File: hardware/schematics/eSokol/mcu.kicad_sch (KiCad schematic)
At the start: 12 parts, among them J1 DB25, J2 to HC-05, SW1 SW_LITTLE, U2 YAAJ_BluePill_SWD_Breakout, U3 TP4056, U9 TCRT5000

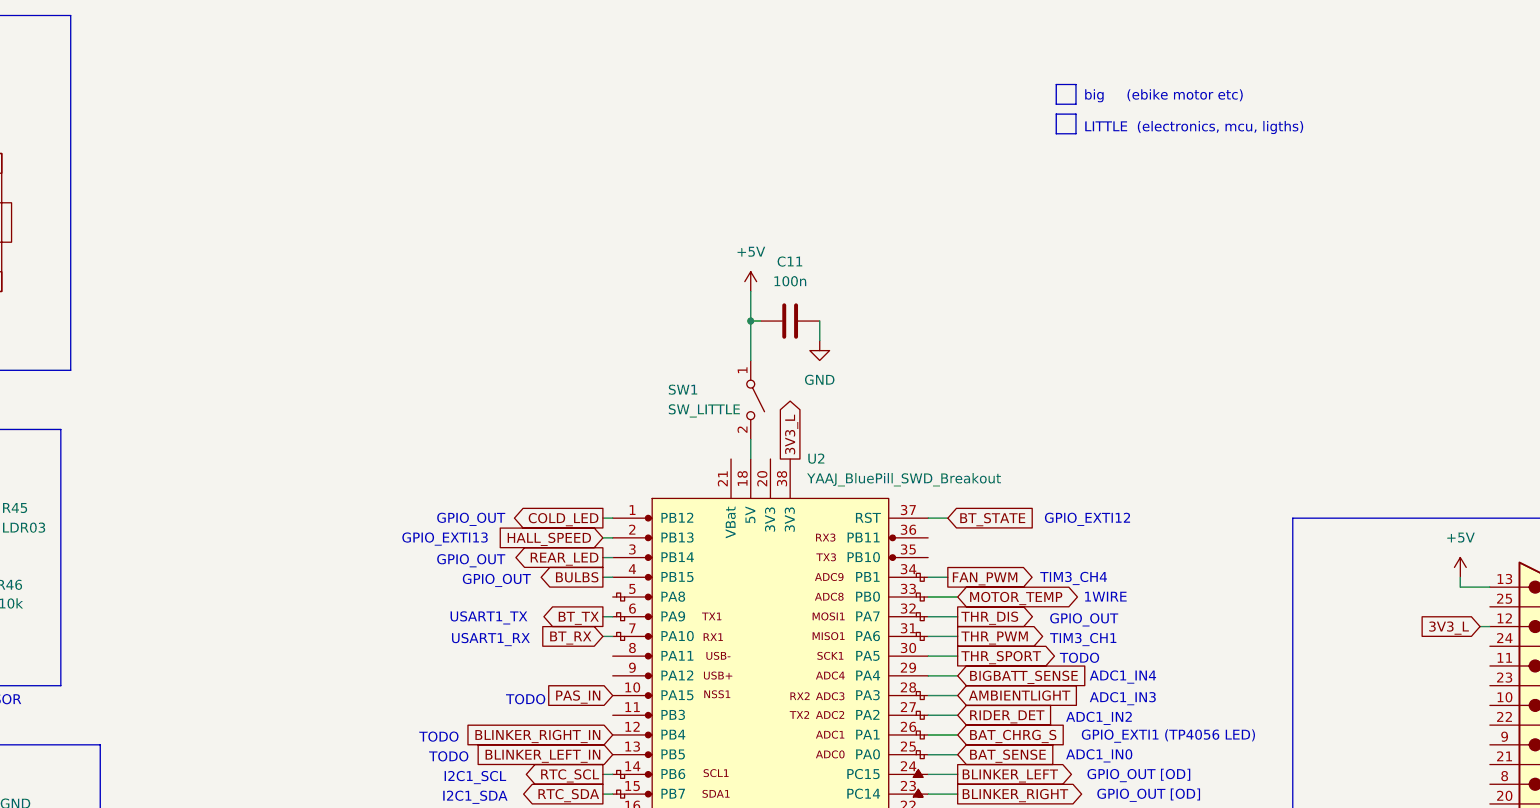
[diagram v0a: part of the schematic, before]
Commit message: WIP: update some schematics to reflect the newest design changes
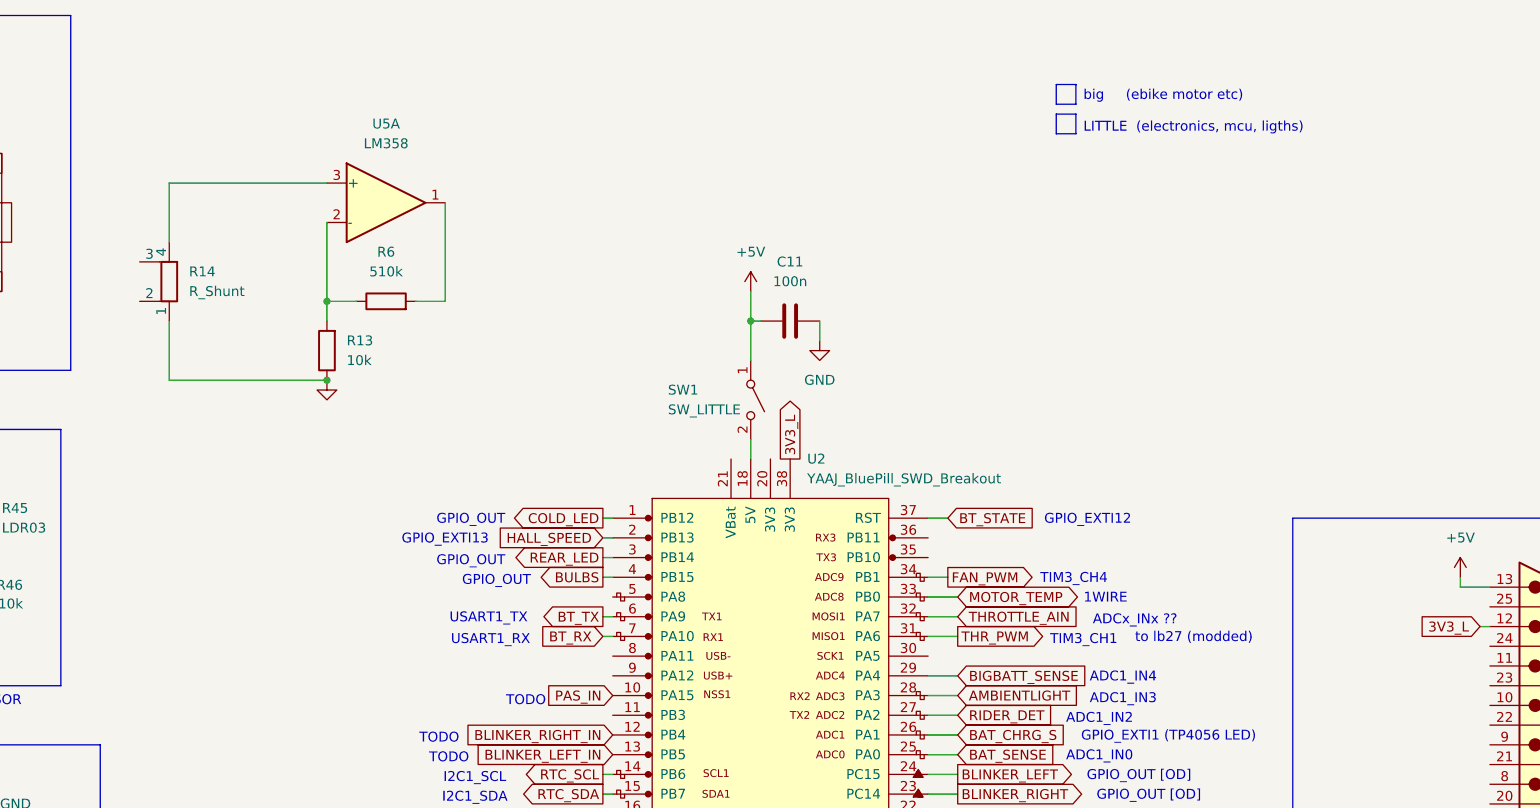
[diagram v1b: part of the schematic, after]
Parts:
- added R13: 10k, symbol Device:R
- added R14: R_Shunt, symbol Device:R_Shunt
- added R6: 510k, symbol Device:R
- added U5: LM358, symbol Amplifier_Operational:LM358
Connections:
- net GND: now also R13.1, R14.1
- net THR_DIS renamed THROTTLE_AIN
- net THR_SPORT: no longer names the net of U2.30 (PA5)
- new net: R14.4, U5.3 (+)
- new net: R13.2, R6.1, U5.2 (-)
- new net: R6.2, U5.1
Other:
- note added: "ADCx_INx ??"
- note added: "to lb27 (modded)"
